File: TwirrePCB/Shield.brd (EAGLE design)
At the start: 96.2 x 53.3 mm, 55 parts, among them Q1 BSS138, Q2 BSS138, T2 BC847, U1 ARDUINO-MEGAPRO

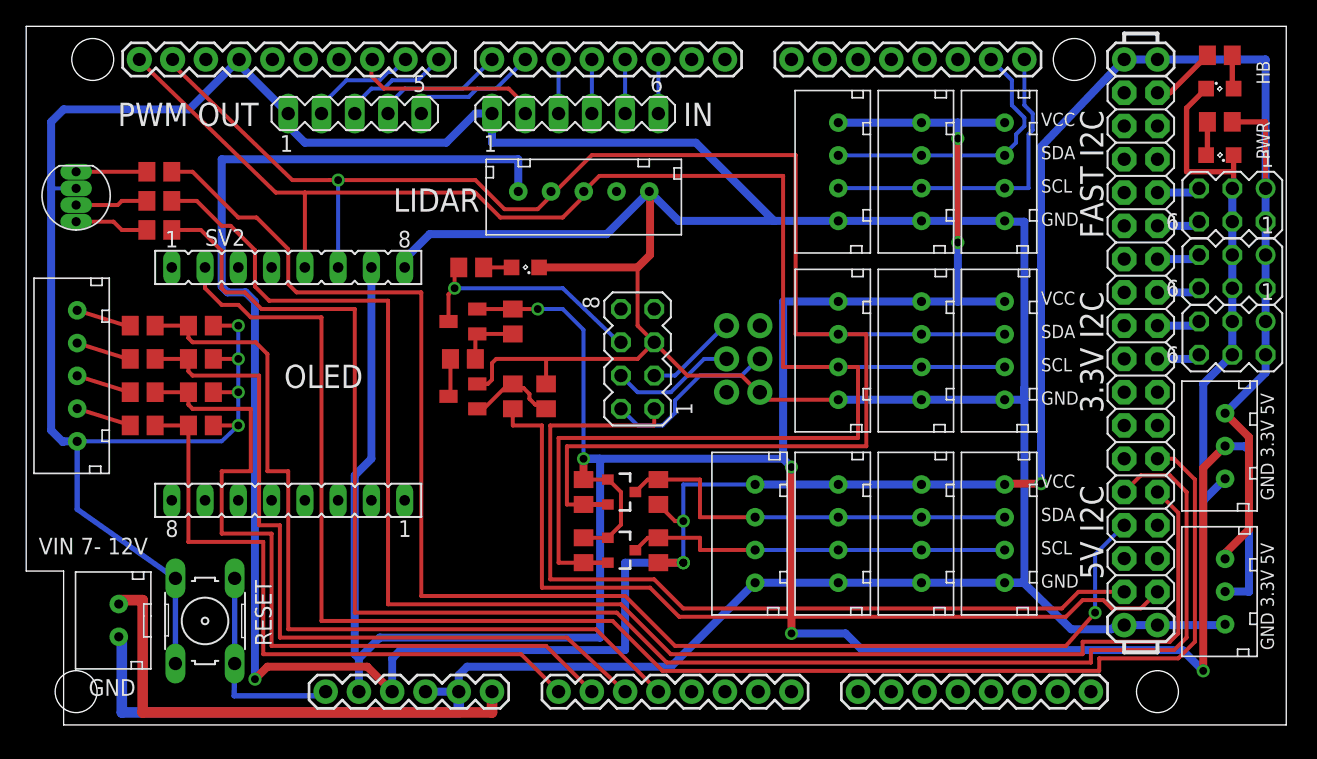
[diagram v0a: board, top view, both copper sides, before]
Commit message: Add caps and lots of other stuff
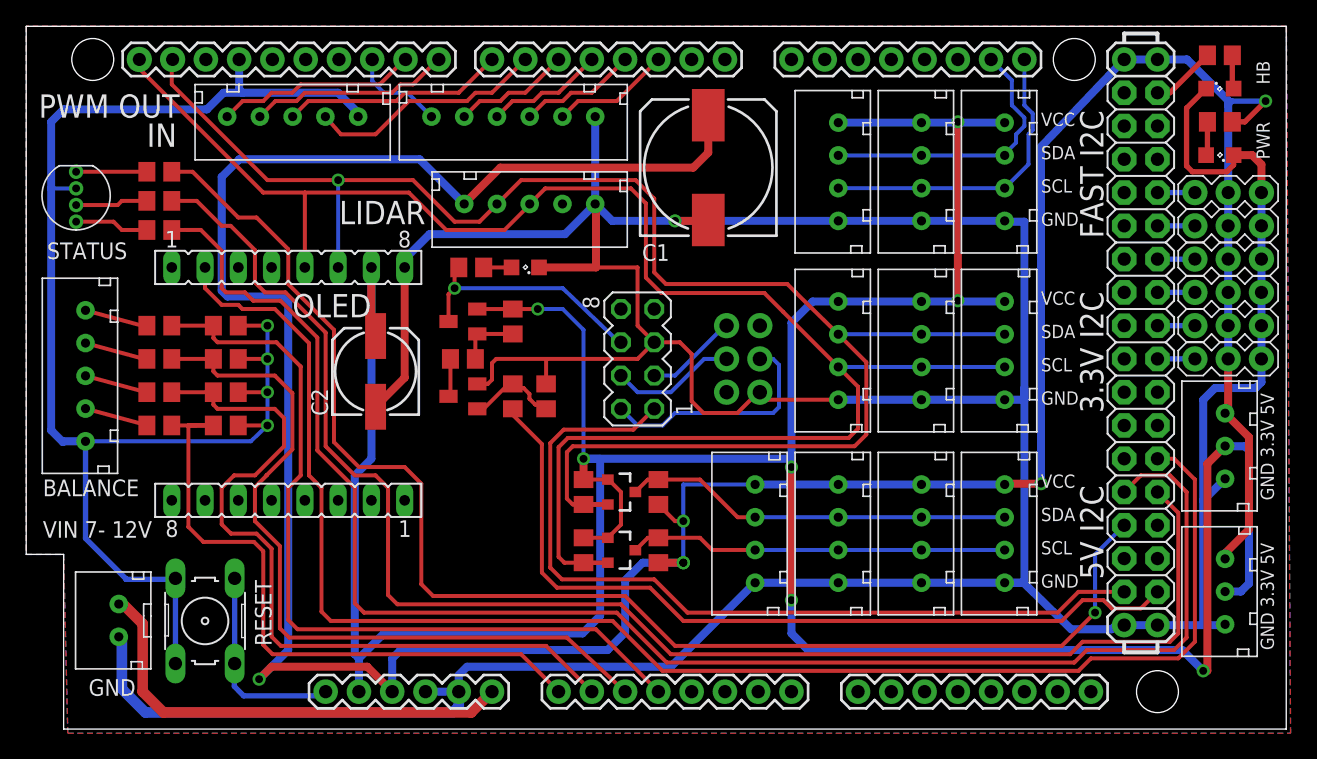
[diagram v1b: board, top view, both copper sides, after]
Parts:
- removed SV1: PWM IN, con-lstb:MA06-1
- removed SV14: PWM OUT, con-lstb:MA05-1
- removed SV4, SV5, SV6: (no value), con-lstb:MA03-2
- added C1: 560uF, resistor:153CLV-1010
- added C2: (no value), resistor:153CLV-0605
- added U$17: JST-6, Arduino-Boards:JST-6
- added U$18: JST-5, Arduino-Boards:JST-5
- added U$19, U$20, U$21, U$22, U$23, U$24: SERVOHEADER, Arduino-Boards:SERVOHEADER
- R22: value (none) -> 220
- moved U$12 4.24 mm to (38.4, 39.4)
- moved R13 1.91 mm to (14.0, 22.9)
- moved R15 1.91 mm to (14.0, 25.4)
- moved R17 1.91 mm to (14.0, 27.9)
- moved R19 1.91 mm to (14.0, 30.5)
- moved R12 1.27 mm to (8.89, 22.9)
- moved R14 1.27 mm to (8.89, 25.4)
- moved R16 1.27 mm to (8.89, 27.9)
- moved R18 1.27 mm to (8.89, 30.5)
- moved U$13 0.63 mm to (2.86, 25.4)
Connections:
- removed net N$31: SV4.5, U1.29
- new net N$36: U$24.S, U1.29
- net +3V3: now also C2.+
- net +5V: now also C1.+, U$19.+, U$20.+, U$21.+, U$22.+, U$23.+, U$24.+; no longer SV4.1, SV4.2, SV5.1, SV5.2, SV6.1, SV6.2
- net GND: now also C1.-, C2.-, U$17.1, U$18.1, U$19.-, U$20.-, U$21.-, U$22.-, U$23.-, U$24.-; no longer SV1.1, SV14.1, SV4.3, SV4.4, SV5.3, SV5.4, SV6.3, SV6.4
- net N$13: now also U$17.6; no longer SV1.2
- net N$16: now also U$18.2; no longer SV14.5
- net N$17: now also U$18.3; no longer SV14.4
- net N$18: now also U$18.4; no longer SV14.3
- net N$19: now also U$18.5; no longer SV14.2
- net N$25: now also U$21.S; no longer SV5.6
- net N$26: now also U$22.S; no longer SV5.5
- net N$27: now also U$23.S; no longer SV4.6
- net N$28: now also U$19.S; no longer SV6.6
- net N$29: now also U$20.S; no longer SV6.5
- net N$5: now also U$17.5, U1.5; no longer SV1.6, U1.2
- net N$6: now also U$17.4, U1.4; no longer SV1.5, U1.3
- net N$8: now also U$17.3, U1.3; no longer SV1.4, U1.4
- net N$9: now also U$17.2, U1.2; no longer SV1.3, U1.5
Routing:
- net +5V: track 243.8 -> 255.5 mm, vias 5 -> 6
- net SDA_LS: track 137.0 -> 126.7 mm
- net N$16: track 10.2 -> 18.2 mm
- net GND: track 441.9 -> 433.9 mm, vias 4 -> 5
- net N$13: track 14.6 -> 7.30 mm
- net N$17: track 10.0 -> 17.0 mm
- net N$18: track 8.50 -> 15.5 mm
- net N$19: track 8.50 -> 15.4 mm
- net SCL_LS: track 137.8 -> 130.9 mm
- net N$9: track 4.13 -> 9.13 mm
- net N$8: track 4.13 -> 9.09 mm
- net N$6: track 4.13 -> 9.05 mm
- net N$5: track 4.13 -> 9.01 mm
- net N$15: track 119.0 -> 114.6 mm
- net SPI_MOSI: track 13.8 -> 18.2 mm
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- added copper zone on layer 1, net GND
- added copper zone on layer 16, net GND
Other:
- board size 96.2 x 53.3 mm -> 96.2 x 53.6 mm
- board text added: "BALANCE"
- board text added: "STATUS"
